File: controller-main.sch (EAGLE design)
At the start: 26 parts

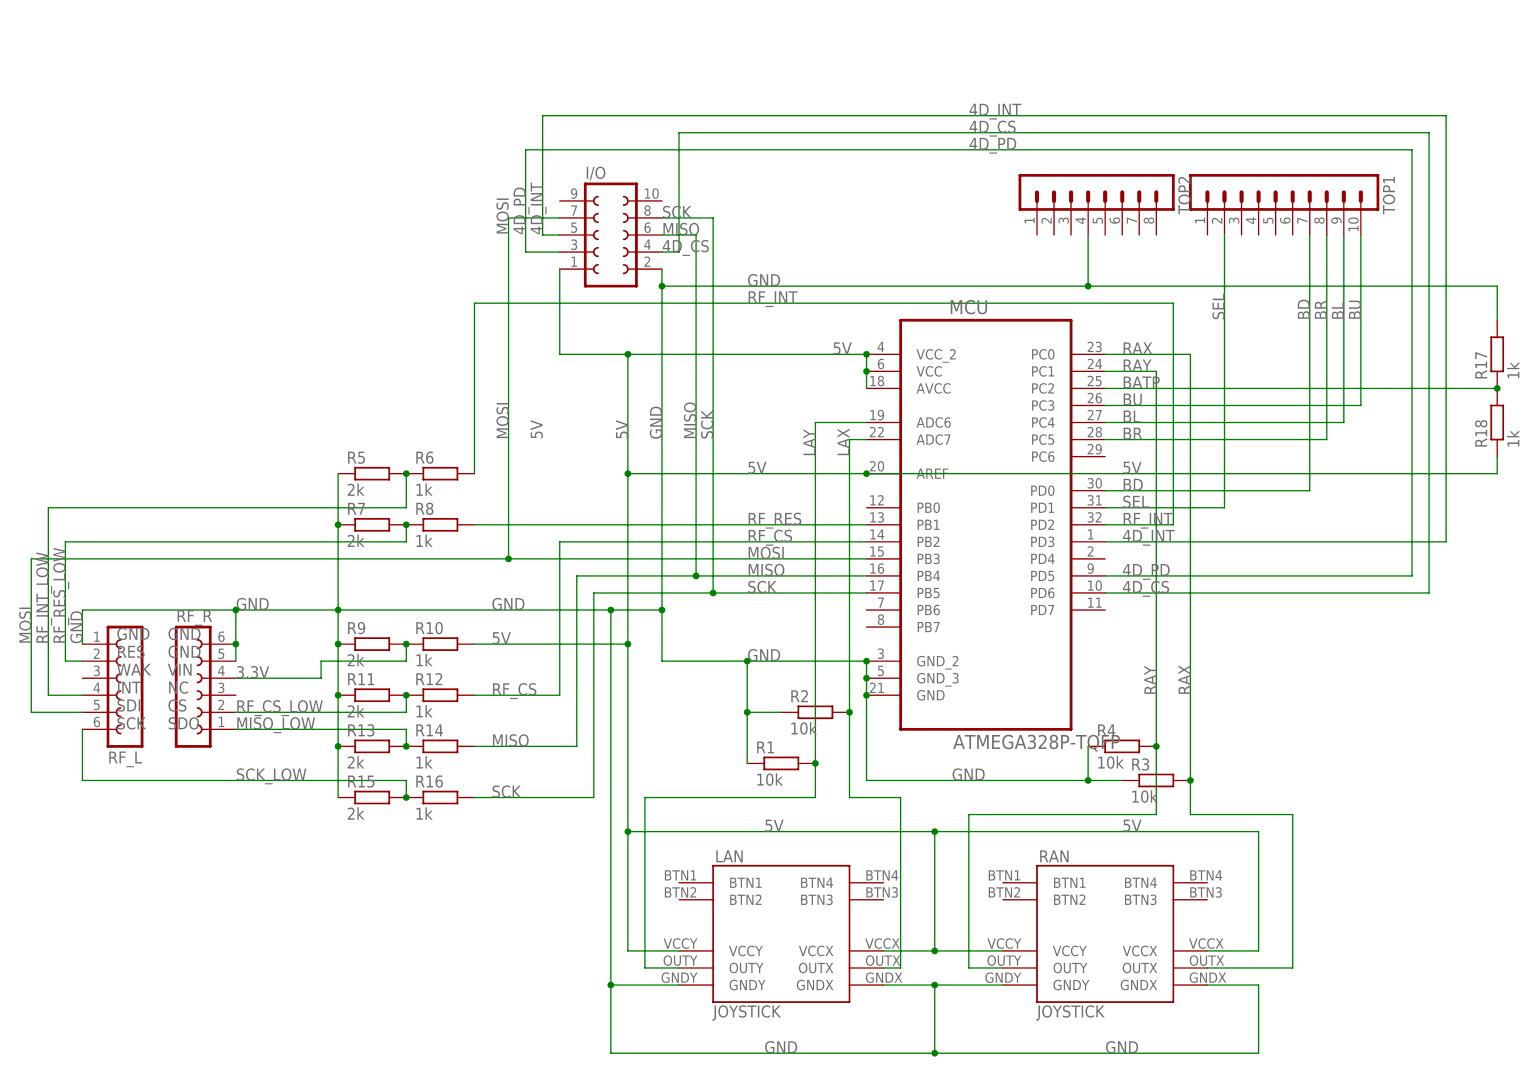
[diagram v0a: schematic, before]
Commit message: only half done
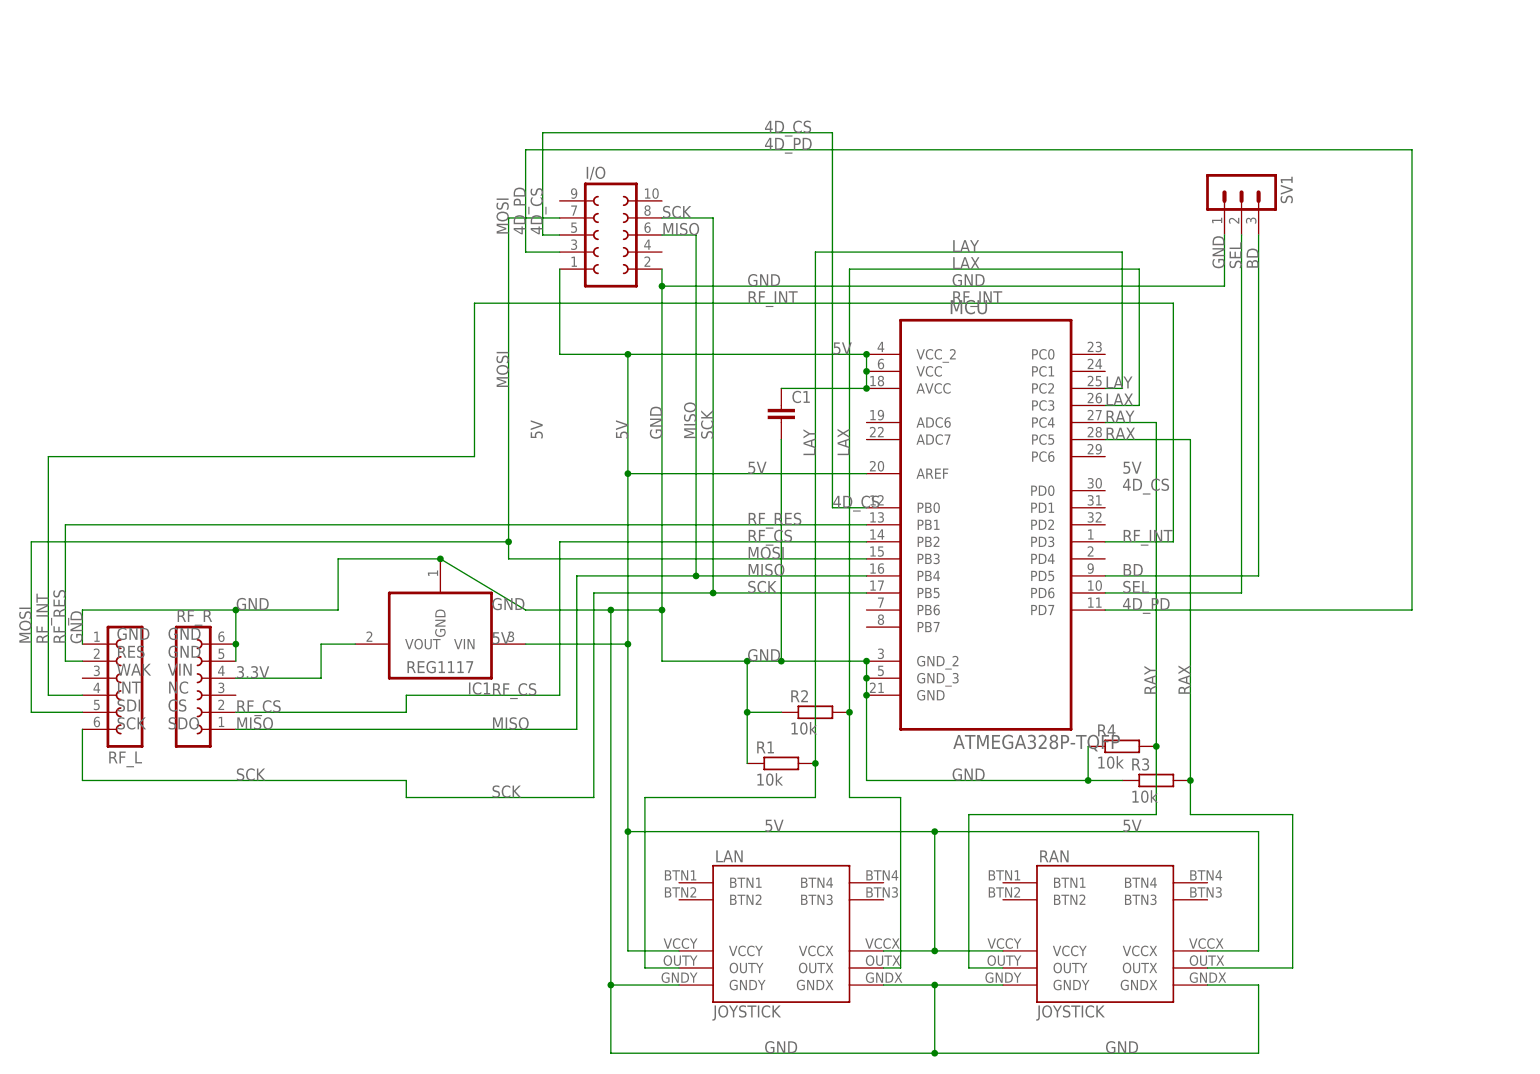
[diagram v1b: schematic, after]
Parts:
- removed R10, R12, R14, R16, R17, R18, R6, R8: 1k, resistor:R-EU_M1206
- removed R11, R13, R15, R5, R7, R9: 2k, resistor:R-EU_M1206
- removed TOP1: (no value), con-lstb:MA10-1W
- removed TOP2: (no value), con-lstb:MA08-1W
- added C1: (no value), resistor:C-EUC1206
- added IC1: REG1117, burr-brown:REG1117
- added SV1: (no value), con-lstb:MA03-1
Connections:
- removed net 4D_INT: I/O.5, MCU.PD3
- removed net BATP: MCU.PC2, R17.1, R18.2
- removed net BL: MCU.PC4, TOP1.9
- removed net BR: MCU.PC5, TOP1.8
- removed net BU: MCU.PC3, TOP1.10
- removed net MISO_LOW: R13.2, R14.1, RF_R.1
- removed net RF_CS_LOW: R11.2, R12.1, RF_R.2
- removed net RF_INT_LOW: R5.2, R6.1, RF_L.4
- removed net RF_RES_LOW: R7.2, R8.1, RF_L.2
- removed net SCK_LOW: R15.2, R16.1, RF_L.6
- net 3.3V: now also IC1.VOUT; no longer R10.1, R9.2
- net 4D_CS: now also I/O.5, MCU.PB0; no longer I/O.4, MCU.PD6
- net 4D_PD: now also MCU.PD7; no longer MCU.PD5
- net 5V: now also C1.1, IC1.VIN; no longer R10.2, R18.1
- net BD: now also MCU.PD5, SV1.3; no longer MCU.PD0, TOP1.7
- net GND: now also C1.2, IC1.GND, SV1.1; no longer R11.1, R13.1, R15.1, R17.2, R5.1, R7.1, R9.1, TOP2.4
- net LAX: now also MCU.PC3; no longer MCU.ADC7
- net LAY: now also MCU.PC2; no longer MCU.ADC6
- net MISO: now also RF_R.1; no longer R14.2
- net RAX: now also MCU.PC5; no longer MCU.PC0
- net RAY: now also MCU.PC4; no longer MCU.PC1
- net RF_CS: now also RF_R.2; no longer R12.2
- net RF_INT: now also MCU.PD3, RF_L.4; no longer MCU.PD2, R6.2
- net RF_RES: now also RF_L.2; no longer R8.2
- net SCK: now also RF_L.6; no longer R16.2
- net SEL: now also MCU.PD6, SV1.2; no longer MCU.PD1, TOP1.2

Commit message: finished the main board
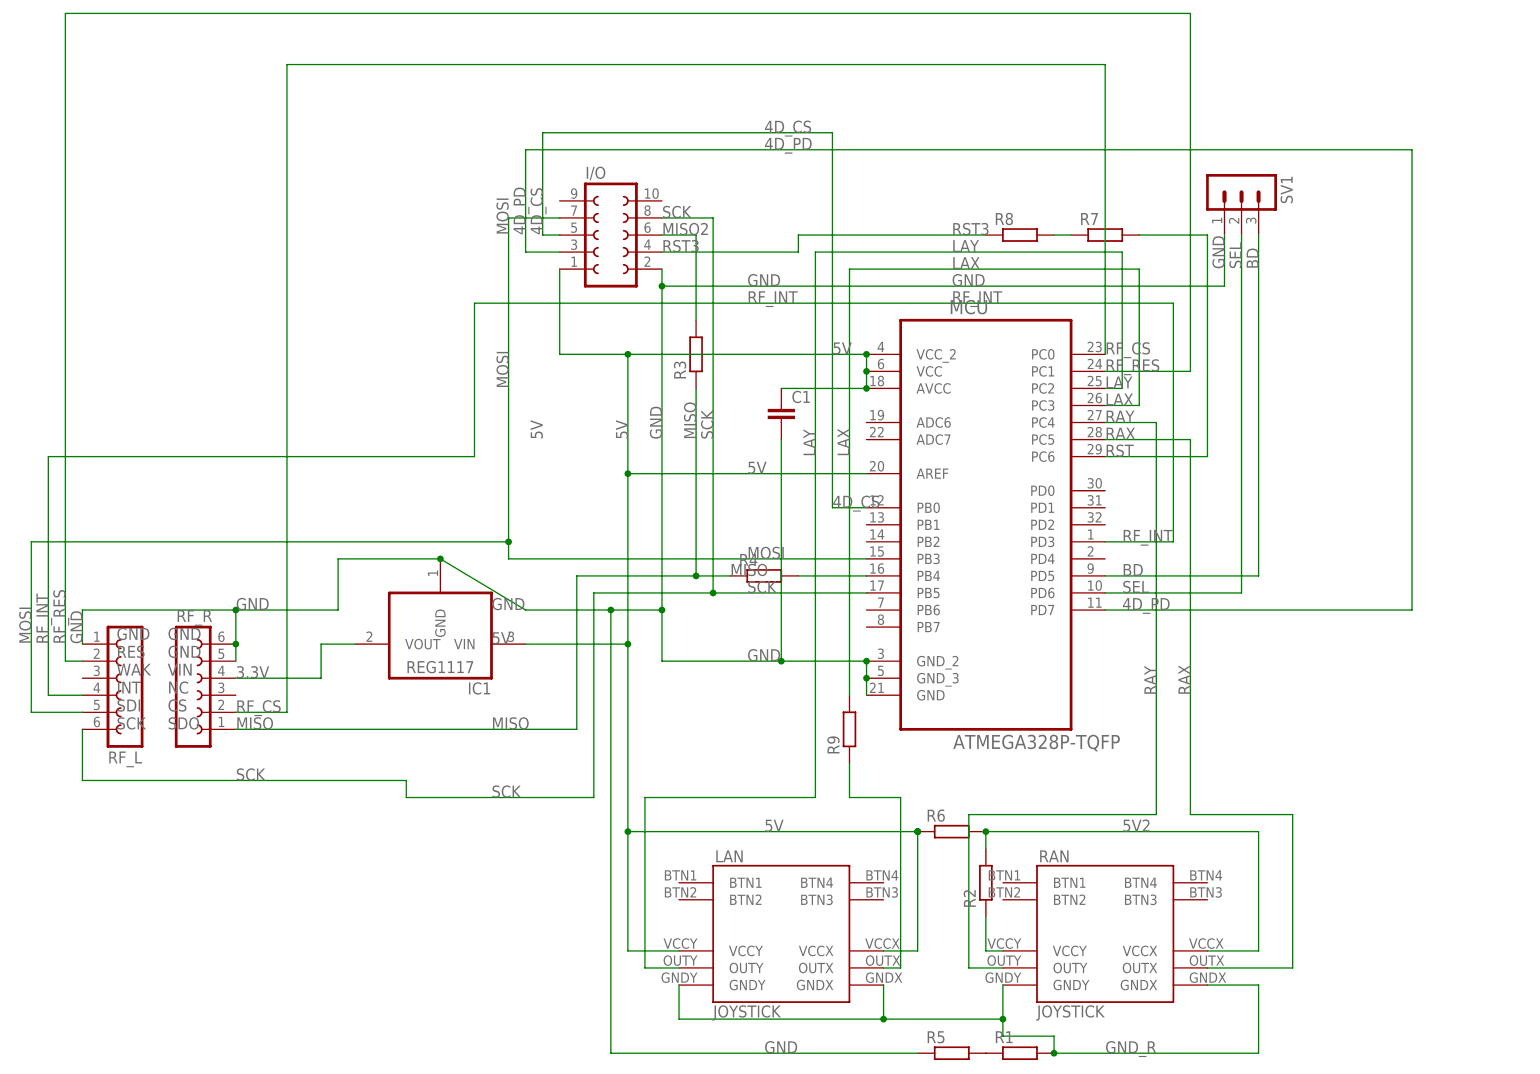
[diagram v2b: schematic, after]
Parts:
- added R5, R6, R7, R8, R9: (no value), resistor:R-EU_M1206
- R1, R2, R3, R4: value 10k -> (none)
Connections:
- new net 5V2: R2.2, R6.2, RAN.VCCX
- new net 5V_R: R2.1, RAN.VCCY
- new net GND_R: LAN.GNDX, LAN.GNDY, R1.2, RAN.GNDX, RAN.GNDY
- new net MISO2: I/O.6, R3.2
- new net MISO3: MCU.PB4, R4.2
- new net N$1: R1.1, R5.2
- new net N$2: LAN.OUTX, R9.1
- new net RST: MCU.PC6, R7.2
- new net RST2: R7.1, R8.2
- new net RST3: I/O.4, R8.1
- net 5V: now also R6.1; no longer RAN.VCCX, RAN.VCCY
- net GND: now also R5.1; no longer LAN.GNDX, LAN.GNDY, R1.1, R2.1, R3.1, R4.1, RAN.GNDX, RAN.GNDY
- net LAX: now also R9.2; no longer LAN.OUTX, R2.2
- net LAY: no longer R1.2
- net MISO: now also R3.1, R4.1; no longer I/O.6, MCU.PB4
- net RAX: no longer R3.2
- net RAY: no longer R4.2
- net RF_CS: now also MCU.PC0; no longer MCU.PB2
- net RF_RES: now also MCU.PC1; no longer MCU.PB1
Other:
- moved on the sheet: R1, R2, R3, R4
